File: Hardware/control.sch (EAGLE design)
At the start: 11 parts, among them IC1 317T

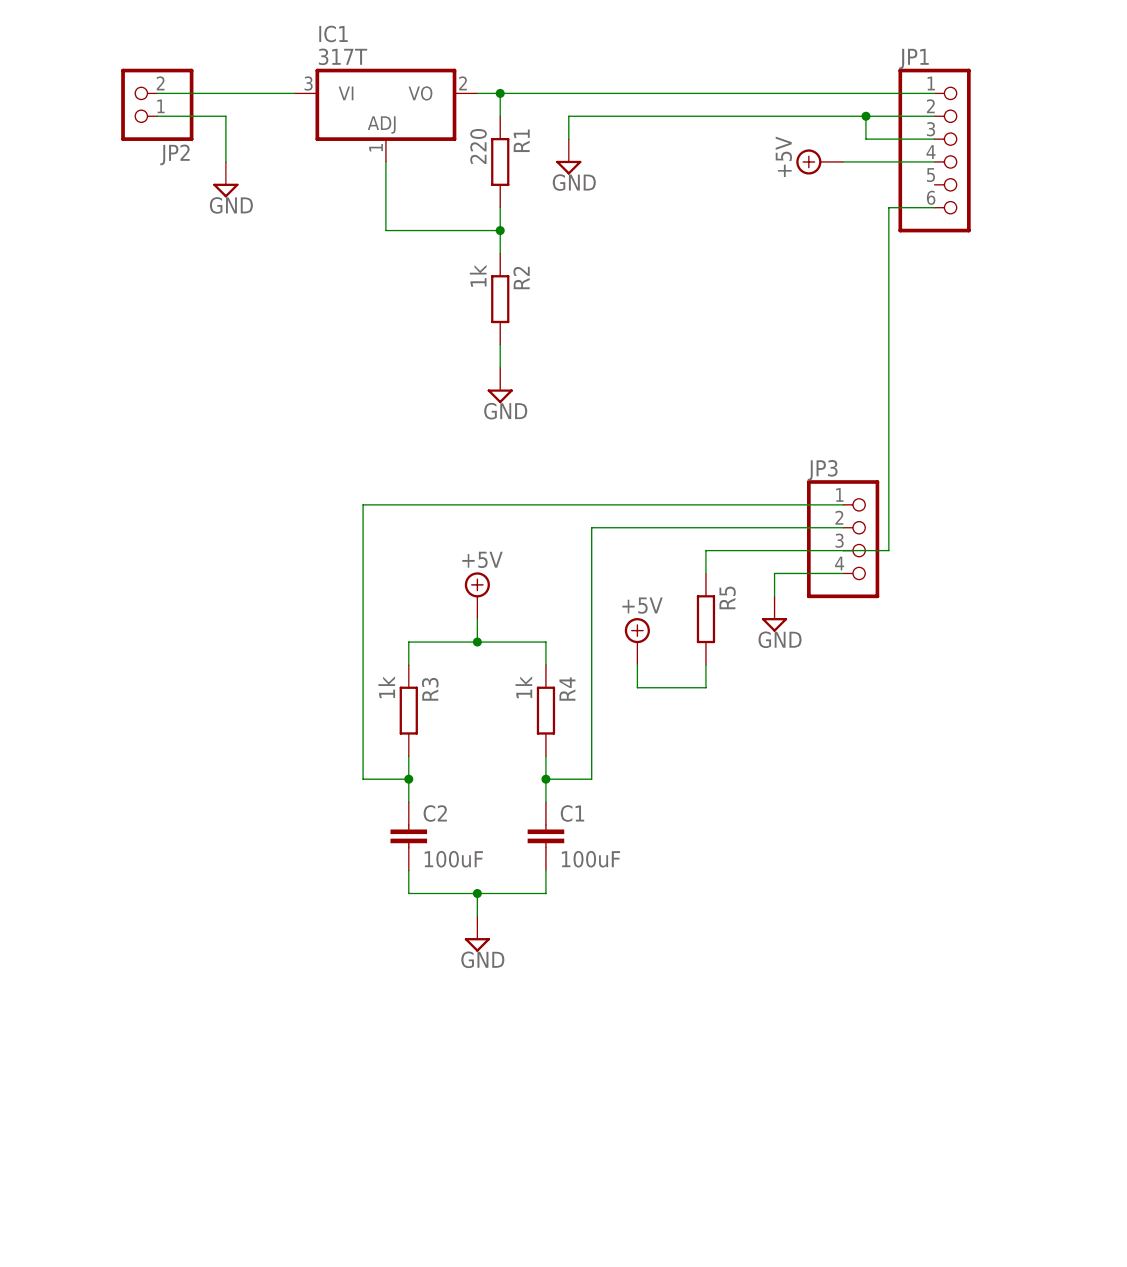
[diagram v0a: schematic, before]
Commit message: Added some better schematics
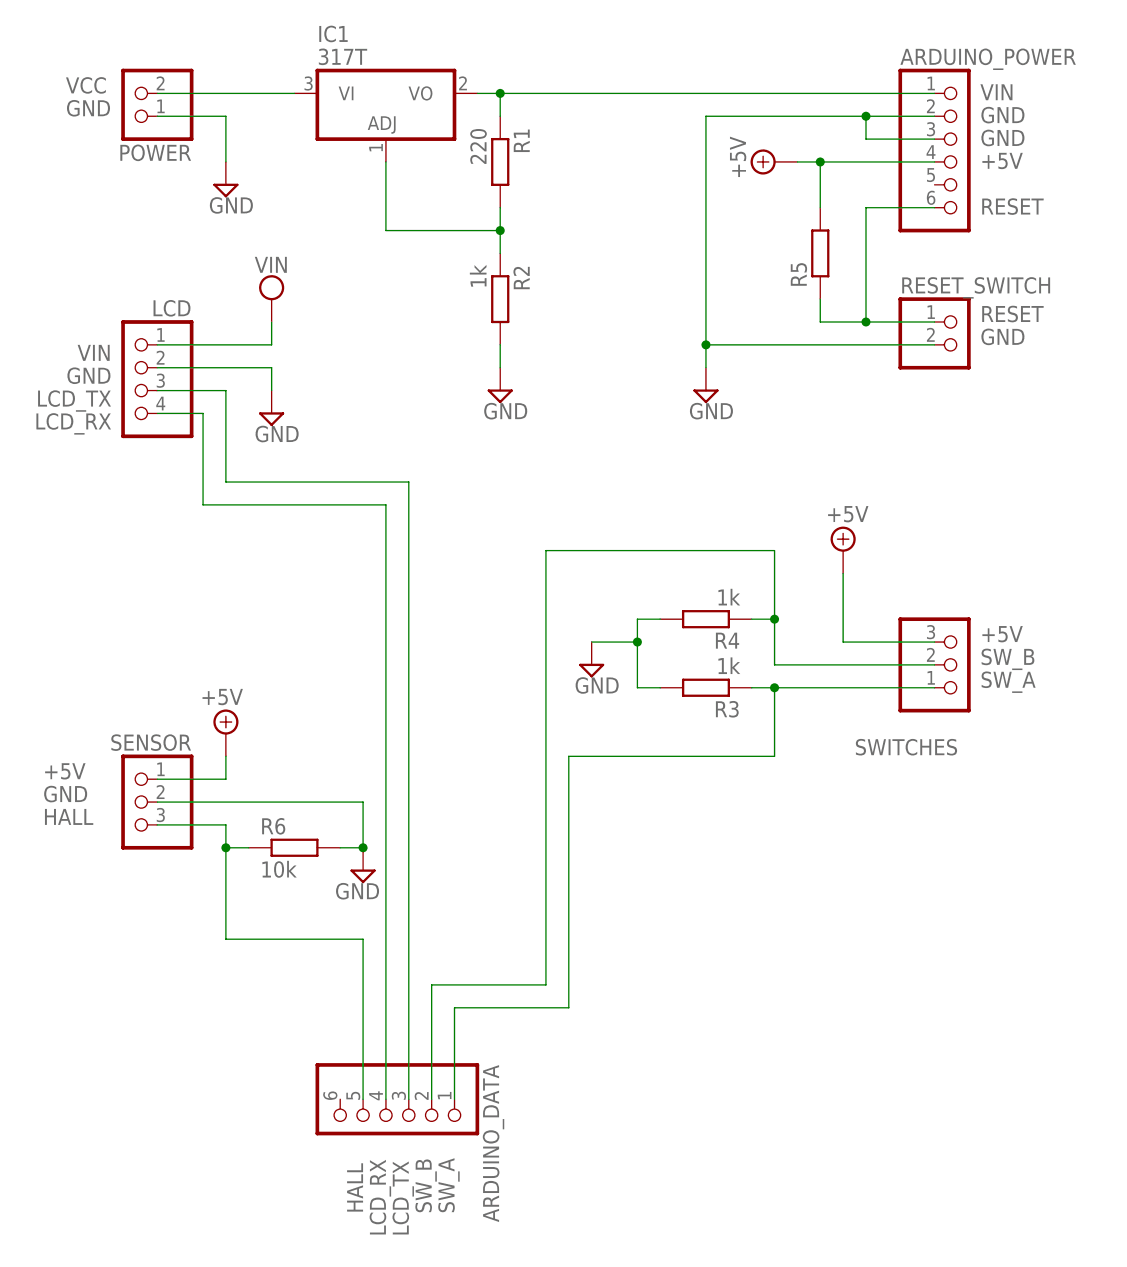
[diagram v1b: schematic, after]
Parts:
- removed C1: 100uF, Rodentometer:C-EU050-024X044
- removed C2: 100uF, Rodentometer:C-EU075-032X103
- removed JP3: (no value), Rodentometer:PINHD-1X4
- added ARDUINO_DATA: (no value), Rodentometer:PINHD-1X6
- added LCD: (no value), Rodentometer:PINHD-1X4
- added R6: 10k, Rodentometer:R-EU_0207/7
- added RESET_SWITCH: (no value), Rodentometer:PINHD-1X2
- added SENSOR, SWITCHES: (no value), Rodentometer:PINHD-1X3
- R3: device Rodentometer:R-EU_0204/7 -> Rodentometer:R-EU_0207/10
- renumbered JP1 to ARDUINO_POWER, JP2 to POWER
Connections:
- net N$2 renamed VCC
- removed net N$1: ARDUINO_POWER.1, IC1.VO, R1.1
- removed net N$3: C2.1, JP3.1, R3.2
- removed net N$4: C1.1, JP3.2, R4.2
- removed net N$6: ARDUINO_POWER.6, JP3.3, R5.1
- new net HALL: ARDUINO_DATA.5, R6.1, SENSOR.3
- new net LCD_RX: ARDUINO_DATA.4, LCD.4
- new net LCD_TX: ARDUINO_DATA.3, LCD.3
- new net RESET: ARDUINO_POWER.6, R5.1, RESET_SWITCH.1
- new net SW_A: ARDUINO_DATA.1, R3.1, SWITCHES.1
- new net SW_B: ARDUINO_DATA.2, R4.1, SWITCHES.2
- new net VIN: ARDUINO_POWER.1, IC1.VO, LCD.1, R1.1
- net +5V: now also SENSOR.1, SWITCHES.3; no longer R3.1, R4.1
- net GND: now also LCD.2, R3.2, R4.2, R6.2, RESET_SWITCH.2, SENSOR.2; no longer C1.2, C2.2, JP3.4
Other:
- moved on the sheet: R3, R4, R5
